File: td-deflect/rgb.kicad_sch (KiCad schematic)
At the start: 83 parts, among them J16 Conn_01x06_Male, J17 Conn_01x06_Male, J5 DB15_Female_HighDensity, J7 Conn_01x08_Male, Q14 BC847, Q15 BC847, Q16 BC847, SW1 SW_DIP_x04, U11 24LC08, U18 M51387P, U19 LMH1980, U20 74LVC1GU04DRLR

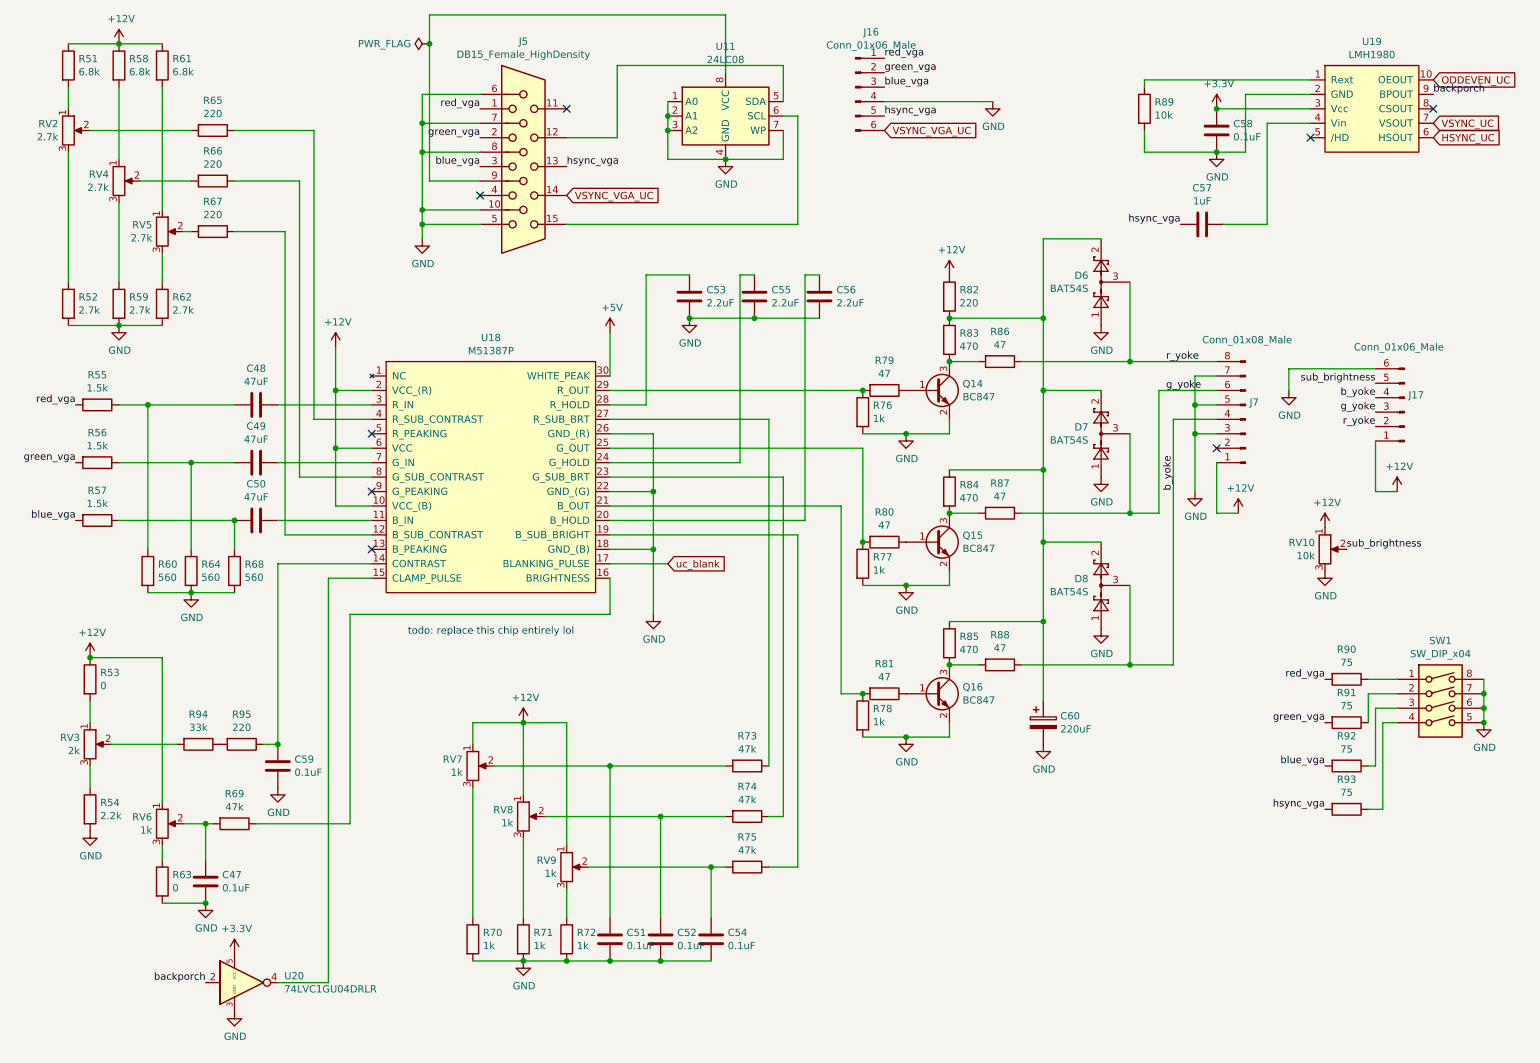
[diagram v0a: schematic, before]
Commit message: more updates
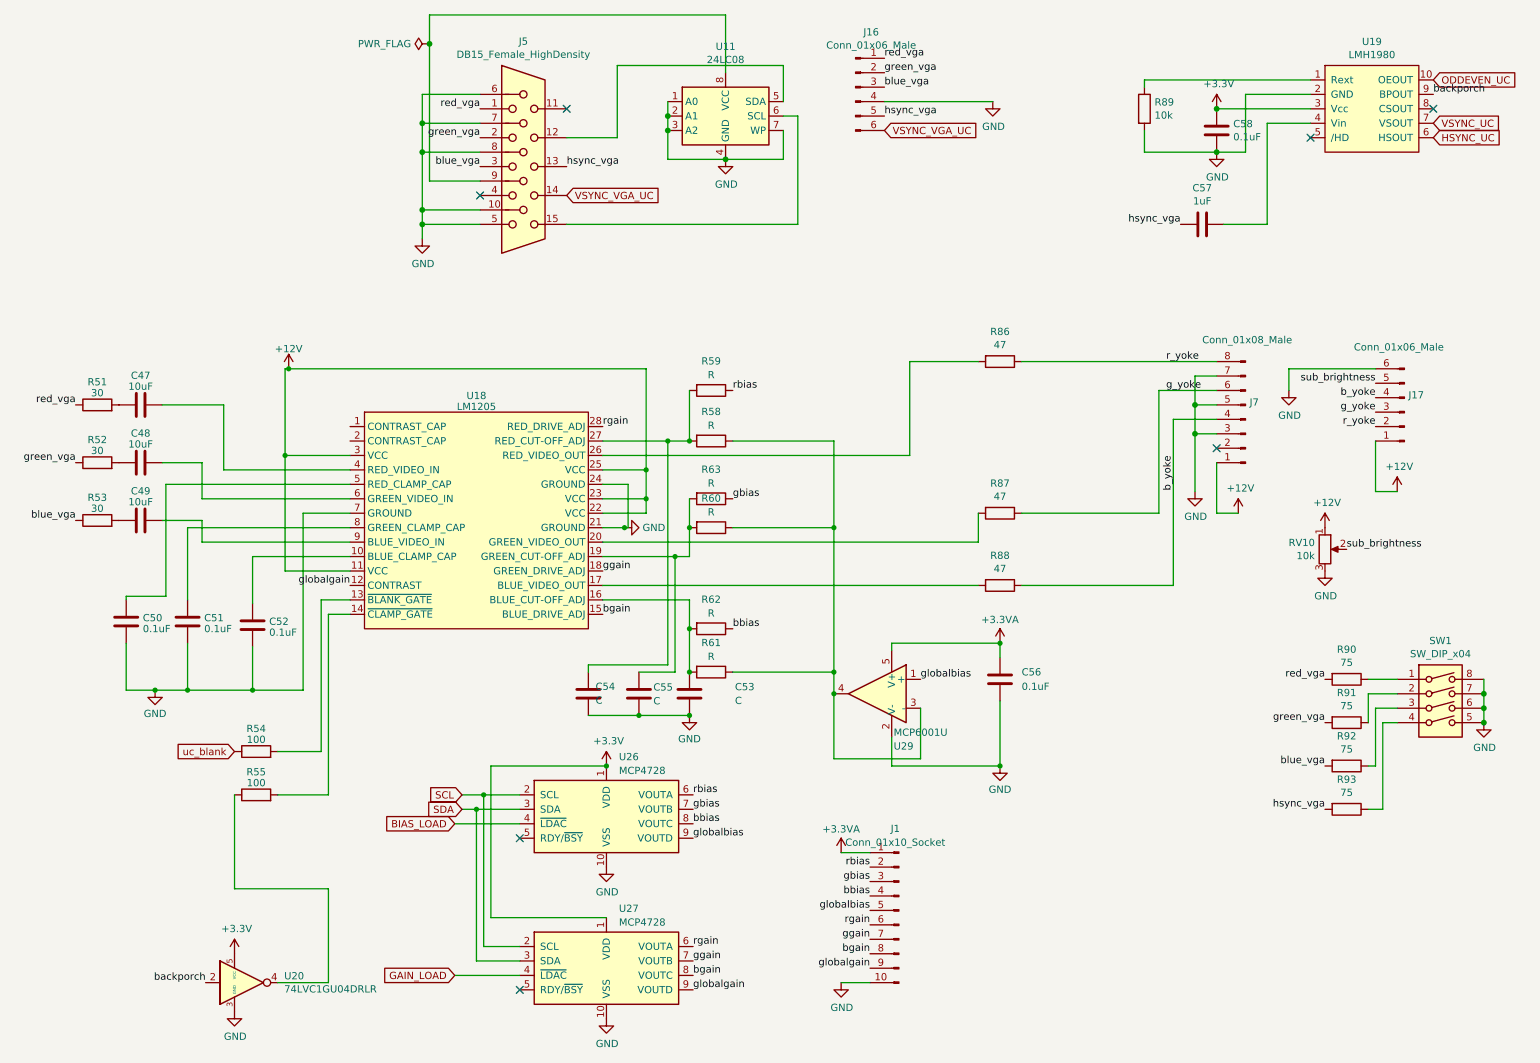
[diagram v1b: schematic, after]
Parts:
- removed C59: 0.1uF, Capacitor_SMD:C_0805_2012Metric_Pad1.15x1.40mm_HandSolder, symbol Device:C
- removed C60: 220uF, Capacitor_THT:CP_Radial_D8.0mm_P3.50mm, symbol Device:CP
- removed D6, D7, D8: BAT54S, Package_TO_SOT_SMD:SOT-23, symbol Diode:BAT54S
- removed Q14, Q15, Q16: BC847, Package_TO_SOT_SMD:SOT-23, symbol Transistor_BJT:BC847
- removed R56, R57: 1.5k, Resistor_SMD:R_0805_2012Metric_Pad1.15x1.40mm_HandSolder, symbol Device:R
- removed R64, R68: 560, Resistor_SMD:R_0805_2012Metric_Pad1.15x1.40mm_HandSolder, symbol Device:R
- removed R65, R66, R67, R82, R95: 220, Resistor_SMD:R_0805_2012Metric_Pad1.15x1.40mm_HandSolder, symbol Device:R
- removed R69, R73, R74, R75: 47k, Resistor_SMD:R_0805_2012Metric_Pad1.15x1.40mm_HandSolder, symbol Device:R
- removed R70, R71, R72, R76, R77, R78: 1k, Resistor_SMD:R_0805_2012Metric_Pad1.15x1.40mm_HandSolder, symbol Device:R
- removed R79, R80, R81: 47, Resistor_SMD:R_0805_2012Metric_Pad1.15x1.40mm_HandSolder, symbol Device:R
- removed R83, R84, R85: 470, Resistor_SMD:R_0805_2012Metric_Pad1.15x1.40mm_HandSolder, symbol Device:R
- removed R94: 33k, Resistor_SMD:R_0805_2012Metric_Pad1.15x1.40mm_HandSolder, symbol Device:R
- removed RV2, RV4, RV5: 2.7k, Potentiometer_THT:Potentiometer_Bourns_3386P_Vertical, symbol Device:R_POT
- removed RV3: 2k, Potentiometer_THT:Potentiometer_Bourns_3386P_Vertical, symbol Device:R_POT
- removed RV6, RV7, RV8, RV9: 1k, Potentiometer_THT:Potentiometer_Bourns_3386P_Vertical, symbol Device:R_POT
- removed U18: M51387P, td-deflect:DIP-30_600_ELL, symbol td-deflect:M51387P
- added J1: Conn_01x10_Socket, symbol Connector:Conn_01x10_Pin
- added U18: LM1205, Package_DIP:DIP-28_W15.24mm, symbol td-crt:LM1205
- added U26, U27: MCP4728, Package_SO:MSOP-10_3x3mm_P0.5mm, symbol Analog_DAC:MCP4728
- added U29: MCP6001U, Package_SO:SOIC-8_3.9x4.9mm_P1.27mm, symbol Amplifier_Operational:MCP6001U
- C47: value 0.1uF -> 10uF; Digikey 1276-1099-1-ND -> (none)
- C48, C49: value 47uF -> 10uF; footprint Capacitor_SMD:C_1206_3216Metric_Pad1.42x1.75mm_HandSolder -> Capacitor_SMD:C_0805_2012Metric_Pad1.15x1.40mm_HandSolder; Digikey 1276-3064-1-ND -> (none); Voltage 6.3V -> (none)
- C50: value 47uF -> 0.1uF; footprint Capacitor_SMD:C_1206_3216Metric_Pad1.42x1.75mm_HandSolder -> Capacitor_SMD:C_0805_2012Metric_Pad1.15x1.40mm_HandSolder; Digikey 1276-3064-1-ND -> (none); Voltage 6.3V -> (none)
- C51, C52: Digikey 1276-1099-1-ND -> (none)
- C53, C55: value 2.2uF -> C; Digikey 1276-2953-1-ND -> (none); Voltage 25V -> (none)
- C54: value 0.1uF -> C; Digikey 1276-1099-1-ND -> (none)
- C56: value 2.2uF -> 0.1uF; Digikey 1276-2953-1-ND -> (none); Voltage 25V -> (none)
- R51: value 6.8k -> 30; Digikey 311-6.80KCRCT-ND -> (none)
- R52: value 2.7k -> 30; Digikey 311-2.70KCRCT-ND -> (none)
- R53: value 0 -> 30; Digikey 311-0.0ARCT-ND -> (none)
- R54: value 2.2k -> 100; Digikey 311-2.20KCRCT-ND -> (none)
- R55: value 1.5k -> 100; Digikey 311-1.50KCRCT-ND -> (none)
- R58, R61: value 6.8k -> R; Digikey 311-6.80KCRCT-ND -> (none)
- R59, R62: value 2.7k -> R; Digikey 311-2.70KCRCT-ND -> (none)
- R60: value 560 -> R; Digikey 311-560CRCT-ND -> (none)
- R63: value 0 -> R; Digikey 311-0.0ARCT-ND -> (none)
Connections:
- net +12V: now also U18.11 (VCC), U18.22 (VCC), U18.23 (VCC), U18.25 (VCC), U18.3 (VCC); no longer R51.1, R53.1, R58.1, R61.1
- net +3V3: now also U26.1 (VDD), U27.1 (VDD)
- net GND: now also C50.1, C51.1, C52.1, J1.10 (Pin_10), U18.21 (GROUND), U18.24 (GROUND), U18.7 (GROUND), U26.10 (VSS), U27.10 (VSS), U29.2 (V-); no longer C47.2, C51.2, C52.2, R52.2, R54.2, R59.2, R60.2, R62.2, R63.2
- net blue_vga: now also R53.1
- net green_vga: now also R52.1
- net red_vga: now also R51.1; no longer R55.2
- net uc_blank: now also R54.1
- net at U20.4: now also R55.1
- net +3.3VA: now reaches C56.1
- net +3.3VA: now also J1.1 (Pin_1), U29.5 (V+)
- net at C55.1: now also R60.2, R63.2, U18.19 (GREEN_CUT-OFF_ADJ)
- net at C53.1: now also R61.2, R62.2, U18.16 (BLUE_CUT-OFF_ADJ)
- net at C48.1: now also R52.2
- net at C49.2: now also U18.9 (BLUE_VIDEO_IN)
- net at C49.1: now also R53.2
- net at C50.2: now also U18.5 (RED_CLAMP_CAP)
- net at R51.2: now also C47.1
- net bbias: now reaches R62.1
- net bbias: now also J1.4 (Pin_4), U26.8 (VOUTC)
- net at R58.2: now also C54.1, R59.2, U18.27 (RED_CUT-OFF_ADJ)
- net rbias: now reaches R59.1
- net rbias: now also J1.2 (Pin_2), U26.6 (VOUTA)
- net gbias: now reaches R63.1
- net gbias: now also J1.3 (Pin_3), U26.7 (VOUTB)
- net at R86.2: now also U18.26 (RED_VIDEO_OUT)
- net at R87.2: now also U18.20 (GREEN_VIDEO_OUT)
- net at R88.2: now also U18.17 (BLUE_VIDEO_OUT)
- new net: C52.2, U18.10 (BLUE_CLAMP_CAP)
- new net: R54.2, U18.13 (~{BLANK_GATE})
- new net: R55.2, U18.14 (~{CLAMP_GATE})
- new net: C47.2, U18.4 (RED_VIDEO_IN)
- new net: C48.2, U18.6 (GREEN_VIDEO_IN)
- new net: C51.2, U18.8 (GREEN_CLAMP_CAP)
- new net: R58.1, R60.1, R61.1, U29.3 (-), U29.4
- new net BIAS_LOAD: U26.4 (~{LDAC})
- new net GAIN_LOAD: U27.4 (~{LDAC})
- new net SCL: U26.2 (SCL), U27.2 (SCL)
- new net SDA: U26.3 (SDA), U27.3 (SDA)
- new net bgain: J1.8 (Pin_8), U18.15 (BLUE_DRIVE_ADJ), U27.8 (VOUTC)
- new net ggain: J1.7 (Pin_7), U18.18 (GREEN_DRIVE_ADJ), U27.7 (VOUTB)
- new net globalbias: J1.5 (Pin_5), U26.9 (VOUTD), U29.1 (+)
- new net globalgain: J1.9 (Pin_9), U18.12 (CONTRAST), U27.9 (VOUTD)
- new net rgain: J1.6 (Pin_6), U18.28 (RED_DRIVE_ADJ), U27.6 (VOUTA)
- no-connect marks 8 -> 7
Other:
- note removed: "todo: replace this chip entirely lol"
- moved on the sheet: R88

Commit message: even more updates
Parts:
- J1: footprint (none) -> Connector_JST:JST_XH_B10B-XH-A_1x10_P2.50mm_Vertical
- SW1: footprint Button_Switch_THT:SW_DIP_SPSTx04_Slide_9.78x12.34mm_W7.62mm_P2.54mm -> Button_Switch_SMD:SW_DIP_SPSTx04_Slide_Omron_A6S-410x_W8.9mm_P2.54mm; Digikey CT2064-ND -> (none)
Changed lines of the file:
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@@
       (effects (font (size 1.27 1.27)))
     )
-    (property "Footprint" "Button_Switch_THT:SW_DIP_SPSTx04_Slide_9.78x12.34mm_W7.62mm_P2.54mm" (at 265.43 137.16 0)
+    (property "Footprint" "Button_Switch_SMD:SW_DIP_SPSTx04_Slide_Omron_A6S-410x_W8.9mm_P2.54mm" (at 265.43 137.16 0)
       (effects (font (size 1.27 1.27)) hide)
     )
@@
       (effects (font (size 1.27 1.27)) hide)
     )
-    (property "Digikey" " CT2064-ND " (at 265.43 137.16 0)
+    (property "Digikey" "" (at 265.43 137.16 0)
       (effects (font (size 1.27 1.27)) hide)
     )
@@
       (effects (font (size 1.27 1.27)))
     )
-    (property "Footprint" "" (at 170.18 172.72 0)
-      (effects (font (size 1.27 1.27)) hide)
-    )
+    (property "Footprint" "Connector_JST:JST_XH_B10B-XH-A_1x10_P2.50mm_Vertical" (at 170.18 172.72 0)
+      (effects (font (size 1.27 1.27)) hide)
+    )
